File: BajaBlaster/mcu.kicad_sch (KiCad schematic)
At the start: 15 parts, among them J1 Conn_01x06_Socket, SW1 SW_Push, SW2 SW_Push, U1 ESP32-WROOM-32, U2 MPU-6050

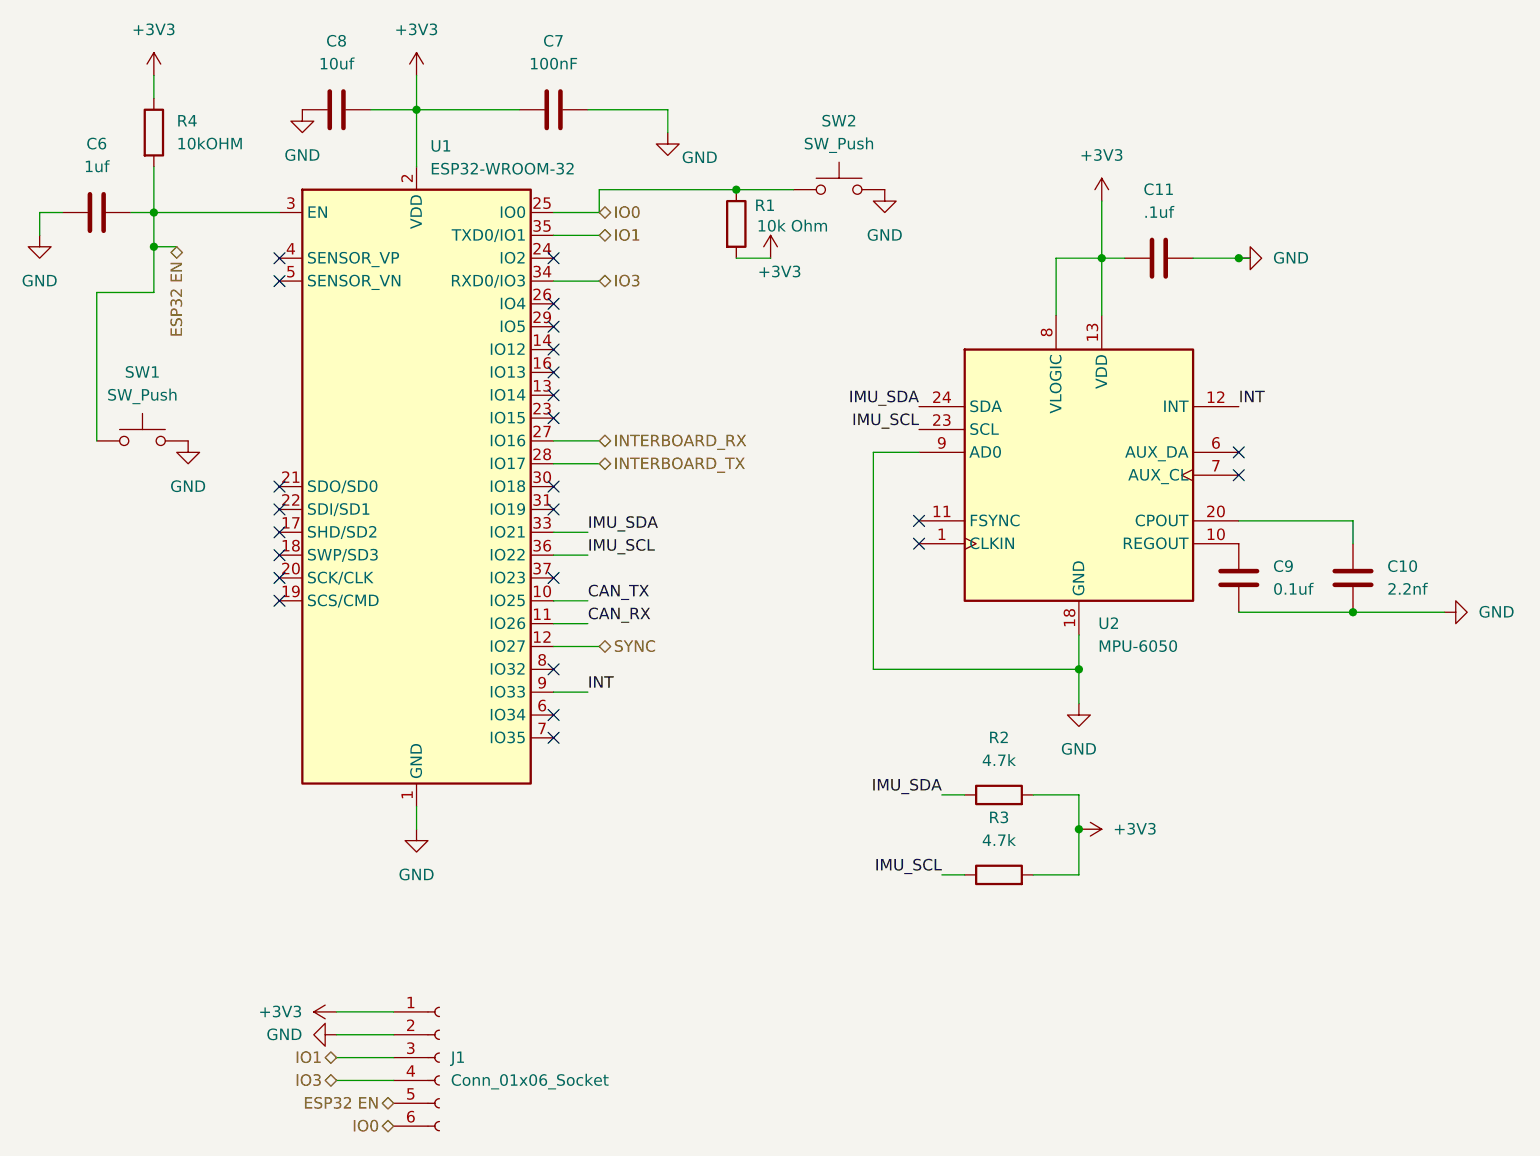
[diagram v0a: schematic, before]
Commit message: added new h tags
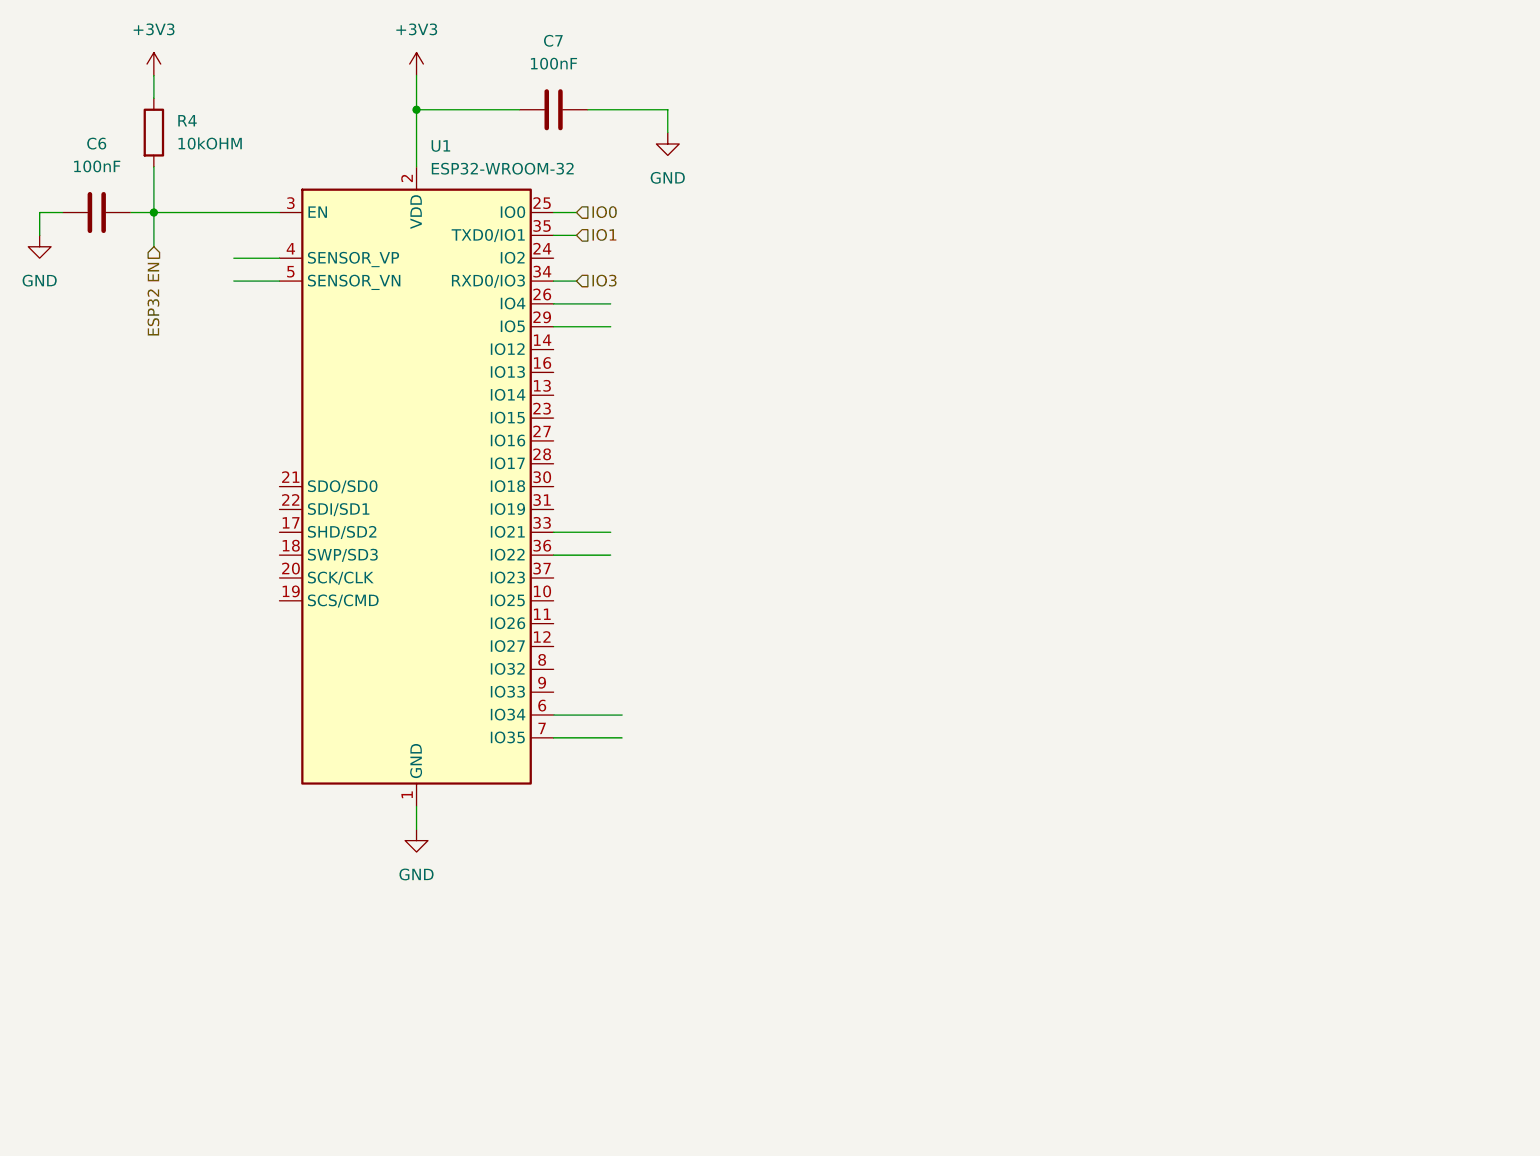
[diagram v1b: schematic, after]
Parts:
- removed C10: 2.2nf, Package_SO:SOIC-8_3.9x4.9mm_P1.27mm, symbol Device:C
- removed C11: .1uf, Package_SO:SOIC-8_3.9x4.9mm_P1.27mm, symbol Device:C
- removed C8: 10uf, Package_SO:SOIC-8_3.9x4.9mm_P1.27mm, symbol Device:C
- removed C9: 0.1uf, Package_SO:SOIC-8_3.9x4.9mm_P1.27mm, symbol Device:C
- removed J1: Conn_01x06_Socket, Connector:Tag-Connect_TC2030-IDC-FP_2x03_P1.27mm_Vertical, symbol Connector:Conn_01x06_Socket
- removed R1: 10k Ohm, Package_DIP:DIP-8_W7.62mm, symbol Device:R
- removed R2, R3: 4.7k, Package_DIP:DIP-8_W7.62mm, symbol Device:R
- removed SW1: SW_Push, Package_DIP:DIP-24_W7.62mm, symbol Switch:SW_Push
- removed SW2: SW_Push, symbol Switch:SW_Push
- removed U2: MPU-6050, Sensor_Motion:InvenSense_QFN-24_4x4mm_P0.5mm, symbol Sensor_Motion:MPU-6050
- C6: value 1uf -> 100nF
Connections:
- net CAN_RX: no longer names the net of U1.11 (IO26)
- net CAN_TX: no longer names the net of U1.10 (IO25)
- net IMU_SCL: no longer names the net of U1.36 (IO22)
- net IMU_SDA: no longer names the net of U1.33 (IO21)
- net INT: no longer names the net of U1.9 (IO33)
- net INTERBOARD_RX: no longer names the net of U1.27 (IO16)
- net INTERBOARD_TX: no longer names the net of U1.28 (IO17)
- net SYNC: no longer names the net of U1.12 (IO27)
- no-connect marks 25 -> 0
